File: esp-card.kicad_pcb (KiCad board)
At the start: 2 copper layers, 6.5 x 10.9 mm, 53 parts, among them J2 Conn_01x04_Socket, U1 NH-B1010RGBT-HF, U2 ESP32-C3FH4, U3 NH-B1010RGBT-HF, U4 TS-1187A-B-A-B, U5 TS-1187A-B-A-B, U58 TS-1187A-B-A-B, U59 YTC-TC16-30, U60 AMS1117-3_3, U61 NH-B1010RGBT-HF, U62 NH-B1010RGBT-HF, U63 NH-B1010RGBT-HF, U64 NH-B1010RGBT-HF, U65 NH-B1010RGBT-HF, U66 NH-B1010RGBT-HF, U67 NH-B1010RGBT-HF, U68 NH-B1010RGBT-HF, U69 NH-B1010RGBT-HF, U70 NH-B1010RGBT-HF, U71 NH-B1010RGBT-HF, U72 NH-B1010RGBT-HF, U73 TS-1187A-B-A-B, X1 CF4040M00015001

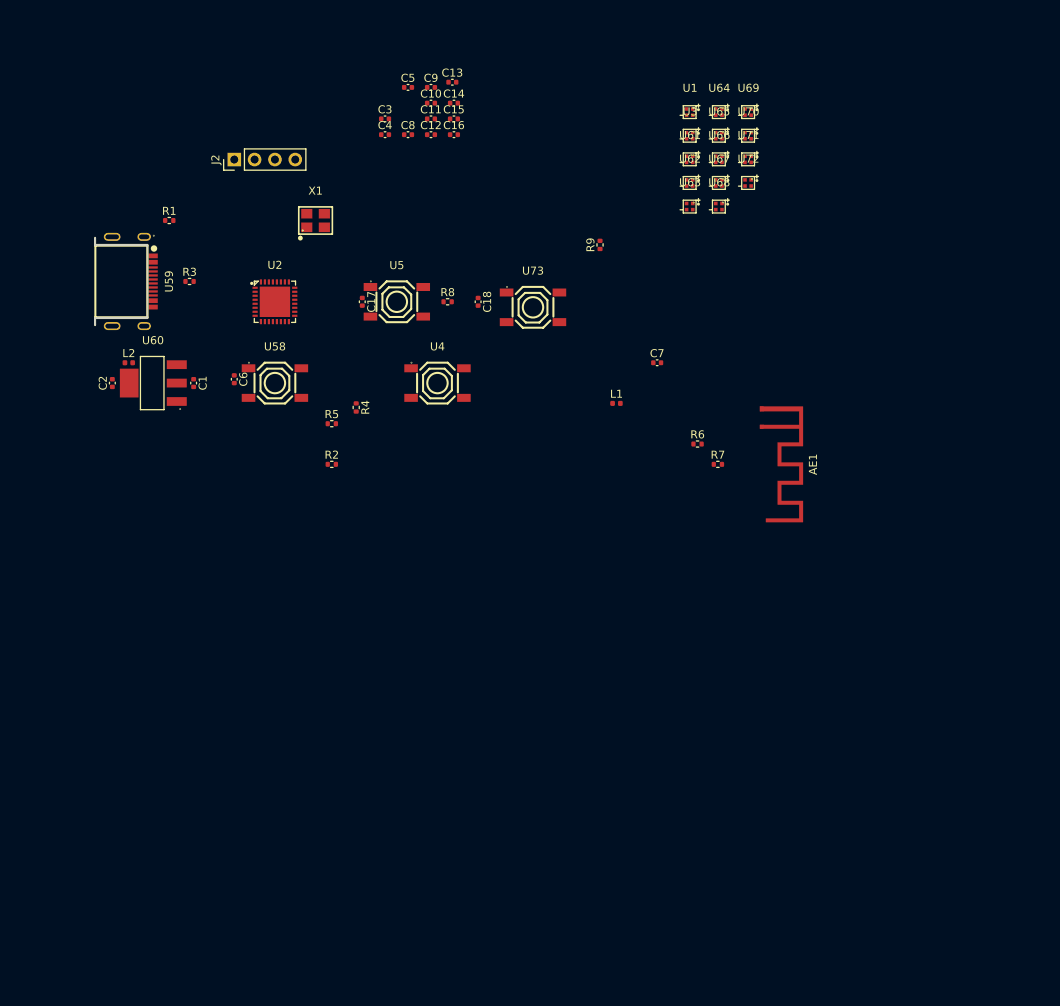
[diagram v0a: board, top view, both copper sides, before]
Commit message: fixed LED matrix
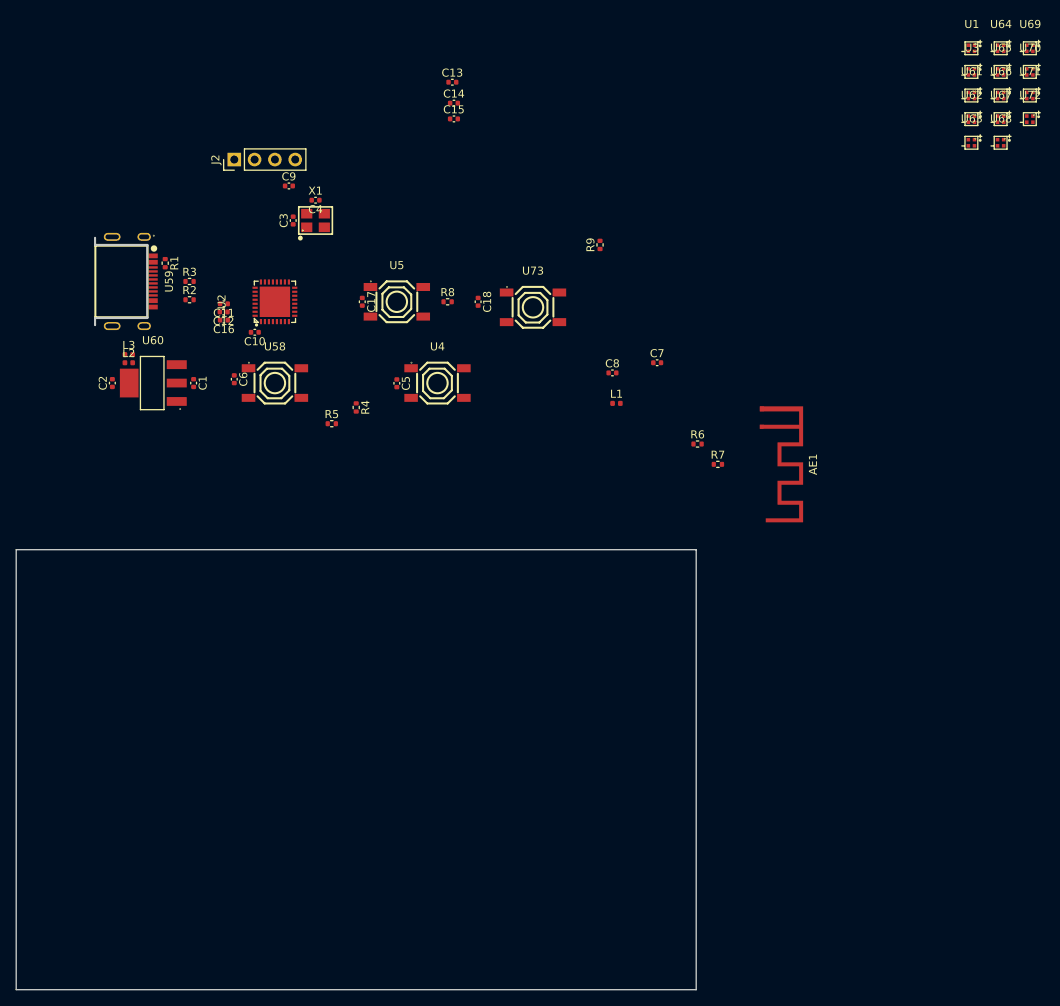
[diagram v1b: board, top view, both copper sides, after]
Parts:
- added L3: 3.9nH, Inductor_SMD:L_0402_1005Metric, F.Cu at (121.4, 95.5)
- L2: value 2nH -> 3.9nH
- moved C8 39.2 mm to (181.9, 97.8)
- moved C5 37.0 mm to (154.9, 99.1), turned to -90 degrees
- moved C16 36.9 mm to (133.3, 91.2), turned to 180 degrees
- moved C10 36.1 mm to (137.2, 92.7), turned to 180 degrees
- moved U64 36.1 mm to (230.4, 57.2)
- moved U65 36.1 mm to (230.4, 60.2)
- moved U66 36.1 mm to (230.4, 63.1)
- moved U67 36.1 mm to (230.4, 66.1)
- moved U68 36.1 mm to (230.4, 69.0)
- moved U69 36.1 mm to (234.1, 57.2)
- moved U70 36.1 mm to (234.1, 60.2)
- moved U71 36.1 mm to (234.1, 63.1)
- moved U72 36.1 mm to (234.1, 66.1)
- moved U1 36.1 mm to (226.8, 57.2)
- moved U3 36.1 mm to (226.8, 60.2)
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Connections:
- C10 pad 1: Net-(C10-Pad1) -> Net-(D2-A)
- L2 pad 2: Net-(C10-Pad1) -> Net-(D2-A)
- U2 pad 10: G5 -> /LED_Matrix_7_pin/CTRL4
- U2 pad 12: G6 -> /LED_Matrix_7_pin/CTRL5
- U2 pad 13: /ESP32/G7 -> /LED_Matrix_7_pin/CTRL6
- U2 pad 2: Net-(C10-Pad1) -> Net-(D2-K)
- U2 pad 3: Net-(C10-Pad1) -> Net-(D2-K)
- U2 pad 31: +3.3V -> Net-(D1-K)
- U2 pad 32: +3.3V -> Net-(D1-K)
- U2 pad 4: G0 -> /LED_Matrix_7_pin/CTRL0
- U2 pad 5: G1 -> /LED_Matrix_7_pin/CTRL1
- U2 pad 8: G3 -> /LED_Matrix_7_pin/CTRL2
- U2 pad 9: G4 -> /LED_Matrix_7_pin/CTRL3
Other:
- board size 6.5 x 10.9 mm -> 85 x 55 mm
